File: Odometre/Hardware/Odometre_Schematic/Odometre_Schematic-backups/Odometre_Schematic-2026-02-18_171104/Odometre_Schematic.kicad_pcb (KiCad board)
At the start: 2 copper layers, 35 parts, among them IC1 STM32C092FCP6, J1 Conn_01x03_Pin, J2 Conn_01x03_Pin, J3 Conn_Alim, J4 Conn_Laser1, J5 Conn_Laser2, J6 Conn_01x06_Pin, J7 Conn_01x06_Pin, SW1 Reset_Botton, SW2 Debug_Botton, U1 MCP2562-E-SN, U2 LM1117DT-3.3, U3 LM1117DT-5.0

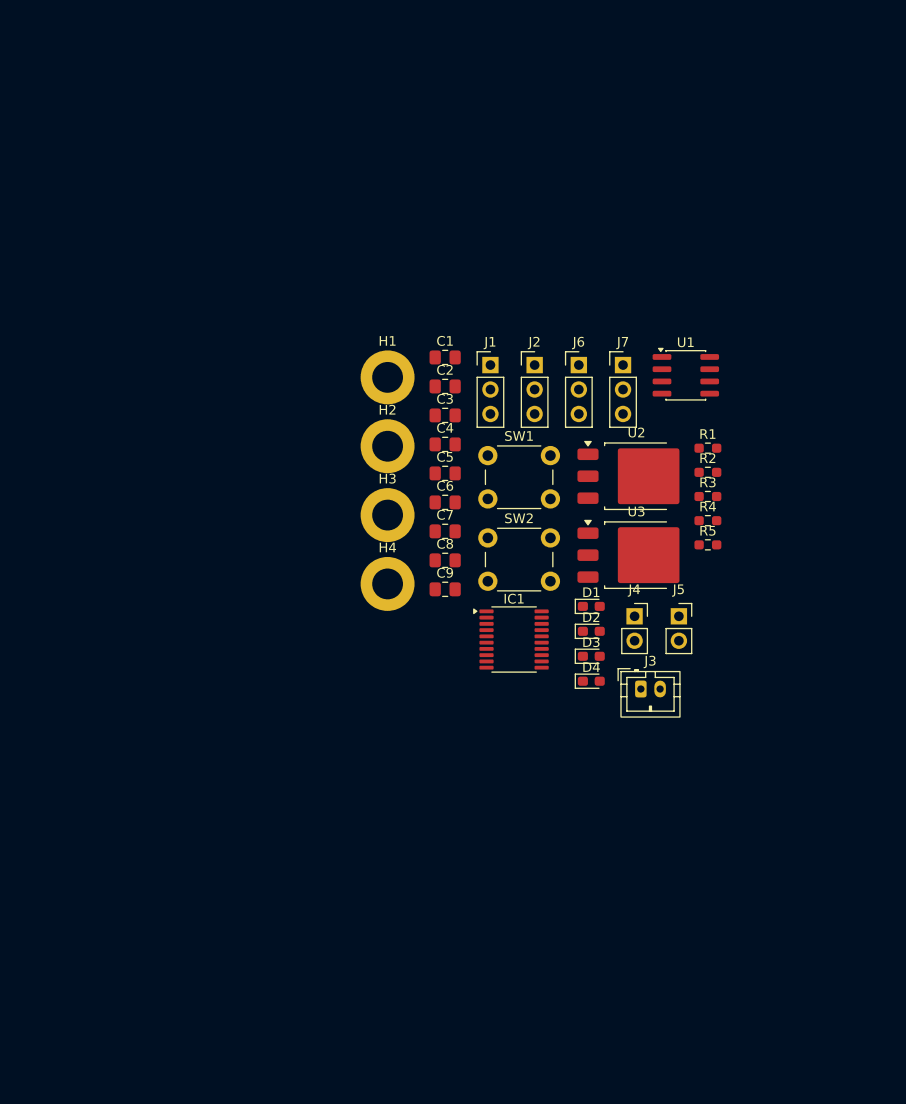
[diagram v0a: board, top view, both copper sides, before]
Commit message: schematic vf
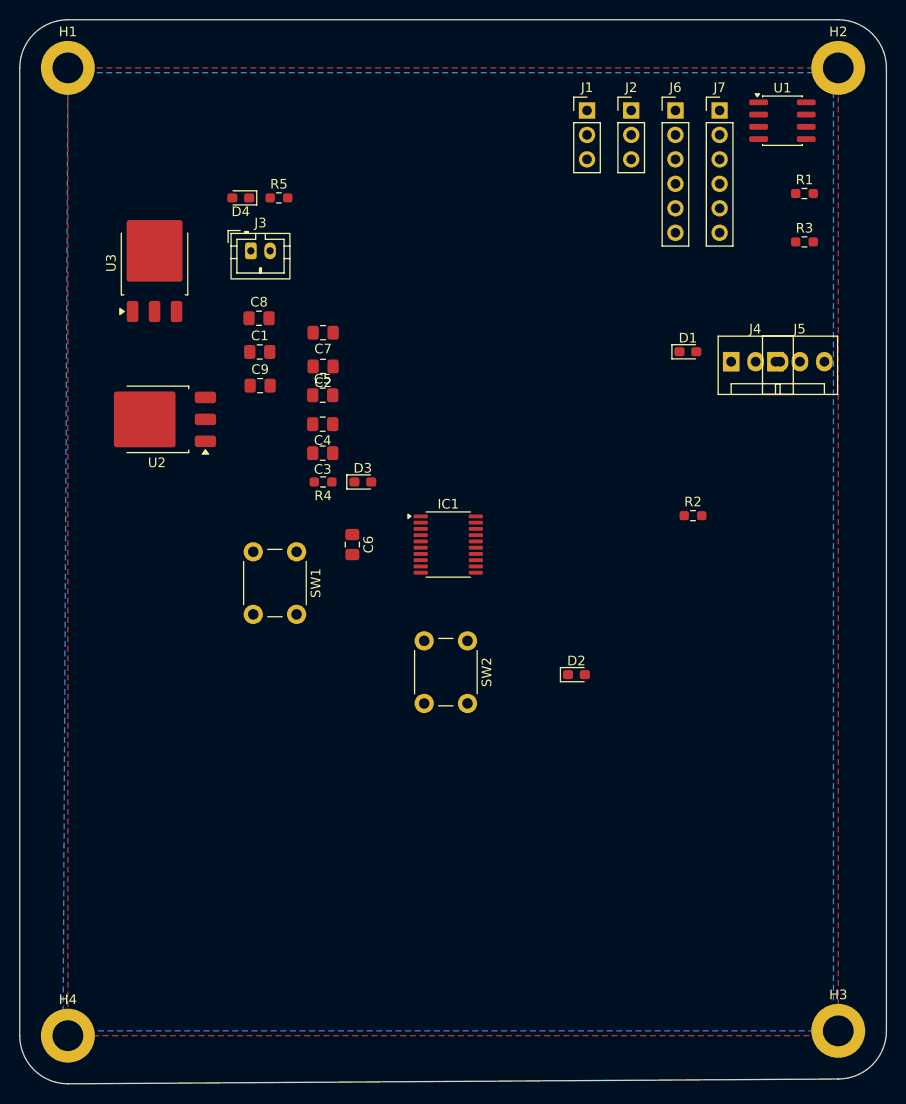
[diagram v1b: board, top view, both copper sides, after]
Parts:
- J4, J5: footprint Connector_PinSocket_2.54mm:PinSocket_1x02_P2.54mm_Vertical -> Connector:FanPinHeader_1x03_P2.54mm_Vertical
- J6, J7: footprint Connector_PinHeader_2.54mm:PinHeader_1x03_P2.54mm_Vertical -> Connector_PinHeader_2.54mm:PinHeader_1x06_P2.54mm_Vertical
- moved H3 71.1 mm to (180.0, 150.0)
- moved D4 62.0 mm to (118.0, 63.5), turned to 180 degrees
- moved H2 61.1 mm to (180.0, 50.0)
- moved J3 60.9 mm to (119.0, 69.0)
- moved U3 58.5 mm to (109.0, 70.3), turned to 90 degrees
- moved H4 57.5 mm to (100.0, 150.5)
- moved R5 57.3 mm to (121.9, 63.5)
- moved U2 50.2 mm to (109.2, 86.5), turned to 180 degrees
- moved H1 46.2 mm to (100.0, 50.0)
- moved R4 40.2 mm to (126.5, 93.0), turned to 180 degrees
- moved C8 31.7 mm to (119.8, 76.0)
- moved D3 29.8 mm to (130.6, 93.0)
- moved C9 28.6 mm to (120.0, 83.0)
- moved R3 28.3 mm to (176.5, 68.1)
- moved D1 28.3 mm to (164.4, 79.5)
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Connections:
- C1 pad 1: ALIM_Trans -> Alim
- C8 pad 1: ALIM_Trans -> Alim
- J3 pad 1: ALIM_Trans -> Alim
- U2 pad 3: ALIM_Trans -> Alim
- U3 pad 3: ALIM_Trans -> Alim
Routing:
- added copper zone on B.Cu, net (none)
- added copper zone on F.Cu, net (none)
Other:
- board outline added: 90 x 110.5 mm
